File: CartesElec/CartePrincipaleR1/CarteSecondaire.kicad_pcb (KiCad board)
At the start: 2 copper layers, 52 x 66 mm, 40 parts, among them Q1 IRLML0030, Q2 IRLML0030, Q3 IRLML0030, Q4 IRLML0030

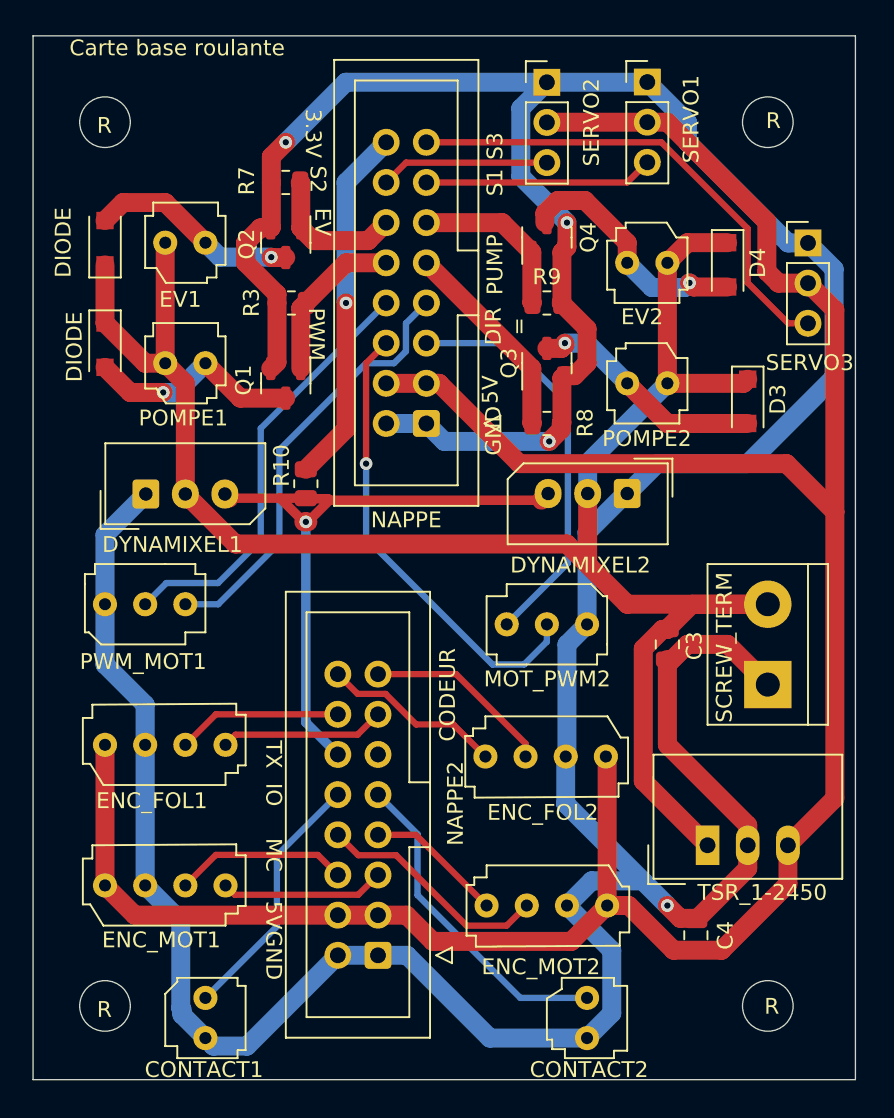
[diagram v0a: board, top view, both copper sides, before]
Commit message: cartePrincipale Update
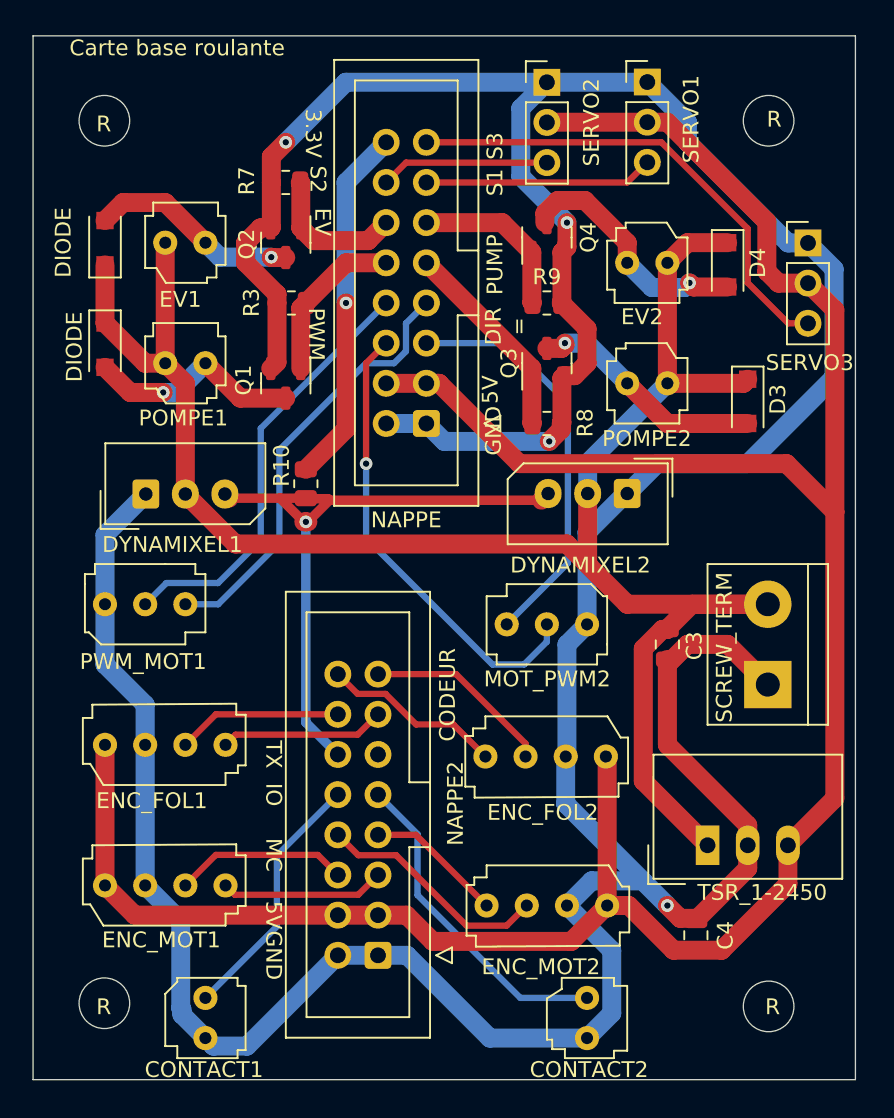
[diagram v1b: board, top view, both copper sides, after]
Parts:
- moved R 0.18 mm to (94.5, 182.1)
- moved R 0.10 mm to (136.5, 126.3)
- moved R 0.10 mm to (94.5, 126.3)
- moved R 0.06 mm to (136.5, 182.3)
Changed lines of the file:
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@@
   )
   (footprint "MountingHole:MountingHole_3.2mm_M3" (layer "F.Cu")
-    (at 94.539011 126.391511)
+    (at 94.5 126.3)
     (descr "Mounting Hole 3.2mm, no annular, M3")
     (tags "mounting hole 3.2mm no annular m3")
@@
   )
   (footprint "MountingHole:MountingHole_3.2mm_M3" (layer "F.Cu")
-    (at 94.539011 182.271511)
+    (at 94.5 182.1)
     (descr "Mounting Hole 3.2mm, no annular, M3")
     (tags "mounting hole 3.2mm no annular m3")
@@
   )
   (footprint "MountingHole:MountingHole_3.2mm_M3" (layer "F.Cu")
-    (at 136.449011 126.391511)
+    (at 136.5 126.3)
     (descr "Mounting Hole 3.2mm, no annular, M3")
     (tags "mounting hole 3.2mm no annular m3")
@@
   )
   (footprint "MountingHole:MountingHole_3.2mm_M3" (layer "F.Cu")
-    (at 136.449011 182.271511)
+    (at 136.5 182.3)
     (descr "Mounting Hole 3.2mm, no annular, M3")
     (tags "mounting hole 3.2mm no annular m3")
